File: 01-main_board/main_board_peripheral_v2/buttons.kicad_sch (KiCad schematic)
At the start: 13 parts, among them U3 NL37WZ14USG

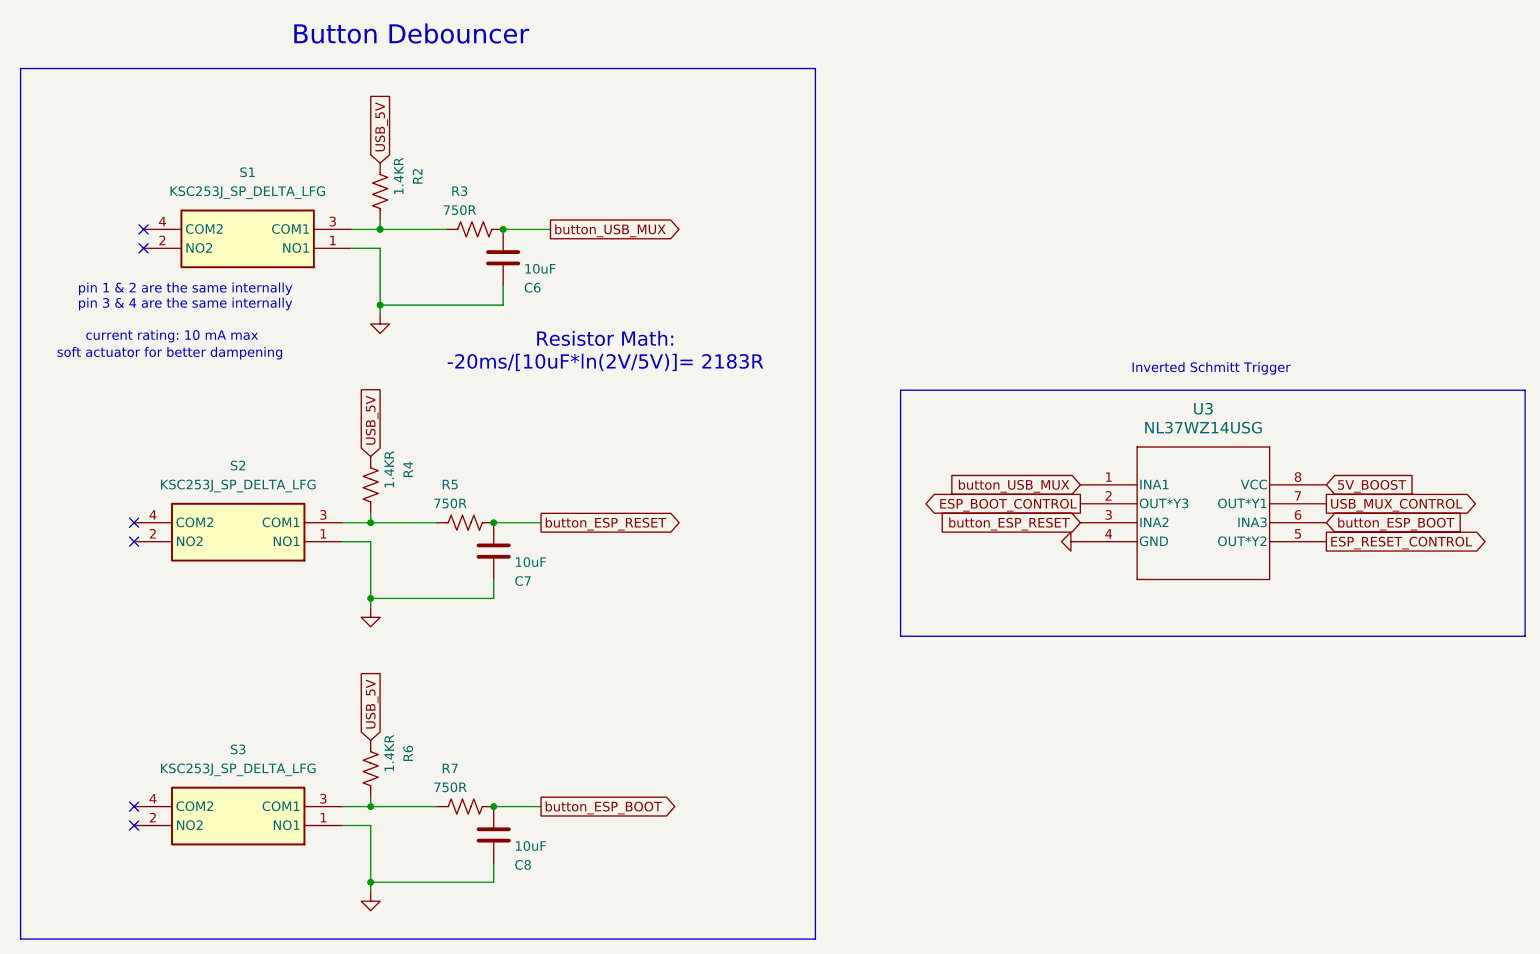
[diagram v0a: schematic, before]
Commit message: Push to change computers. New schematic.
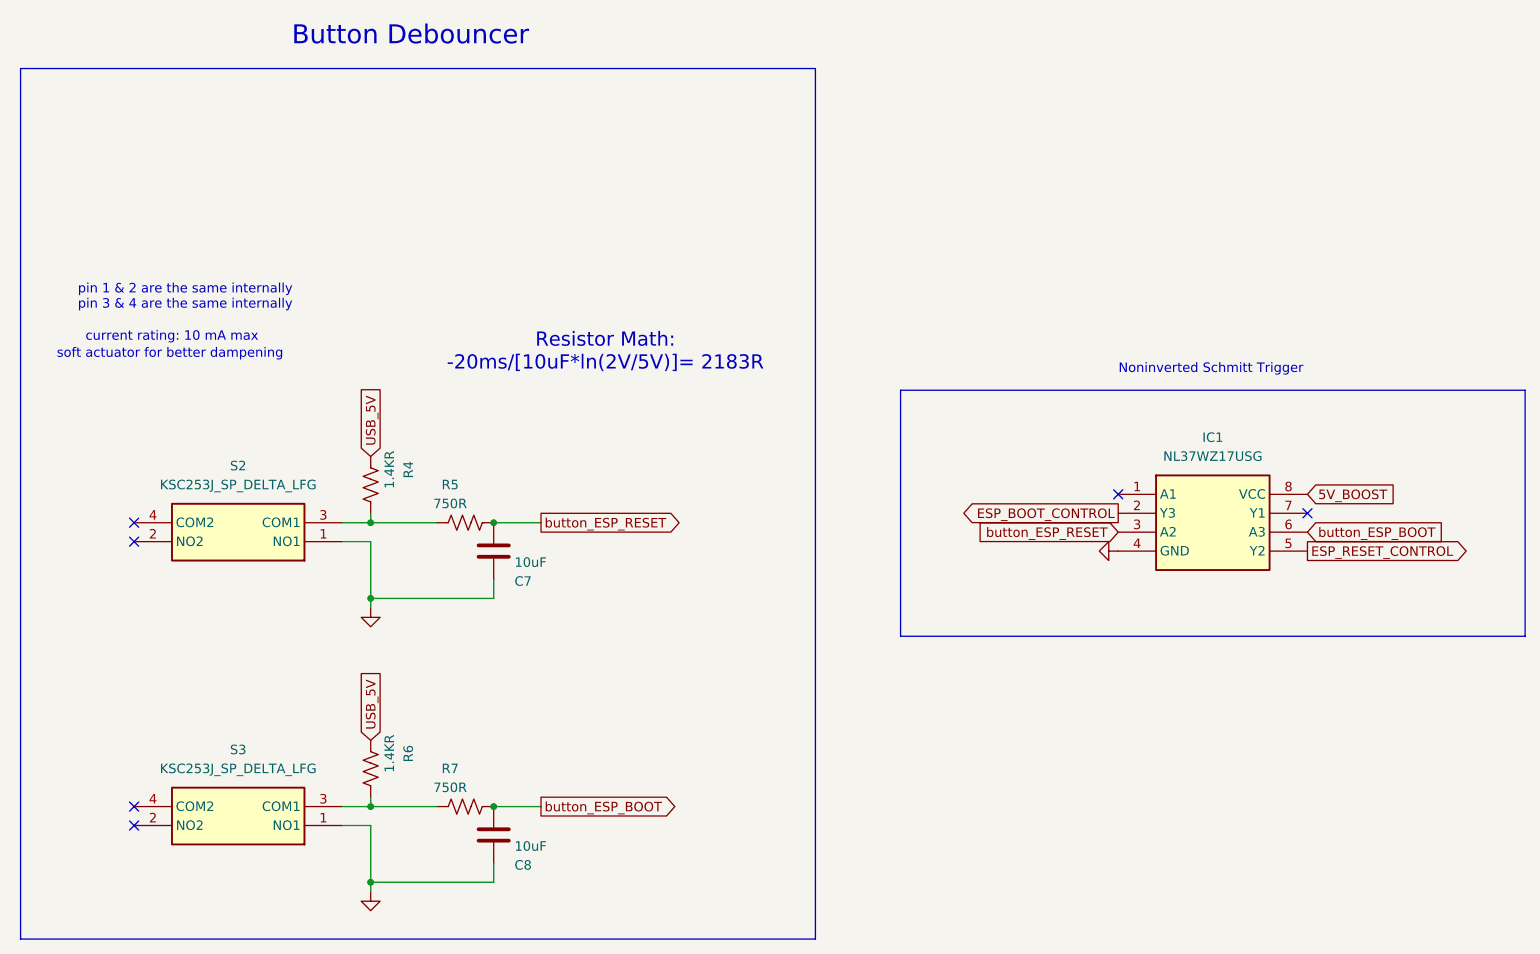
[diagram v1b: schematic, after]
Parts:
- removed C6: 10uF, Capacitor_SMD:C_0603_1608Metric, symbol Device:C
- removed R2: 1.4KR, Resistor_SMD:R_0402_1005Metric, symbol Device:R_US
- removed R3: 750R, Resistor_SMD:R_0402_1005Metric, symbol Device:R_US
- removed S1: KSC253J_SP_DELTA_LFG, 22XT_Main_Peripheral:KSC253JSPDELTALFG, symbol 22XT_Main:KSC253J_SP_DELTA_LFG
- removed U3: NL37WZ14USG, 22XT_Main_Peripheral:NL37WZ14USG, symbol 22XT_Main:NL37WZ14USG
- added IC1: NL37WZ17USG, SOP50P312X90-8N, symbol NL37WZ17USG:NL37WZ17USG
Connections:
- net 5V_BOOST: now also IC1.8 (VCC)
- net ESP_BOOT_CONTROL: now also IC1.2 (Y3)
- net ESP_RESET_CONTROL: now also IC1.5 (Y2)
- net GND: now also IC1.4 (GND)
- net button_ESP_BOOT: now also IC1.6 (A3)
- net button_ESP_RESET: now also IC1.3 (A2)
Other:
- note added: "Noninverted Schmitt Trigger"
- note removed: "Inverted Schmitt Trigger"
